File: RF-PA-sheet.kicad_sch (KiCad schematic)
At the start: 42 parts, among them J7 SMA_F, J8 U.fl, U10 MHW720A, U14 PSA4-5043, U17 B39431B3710U410

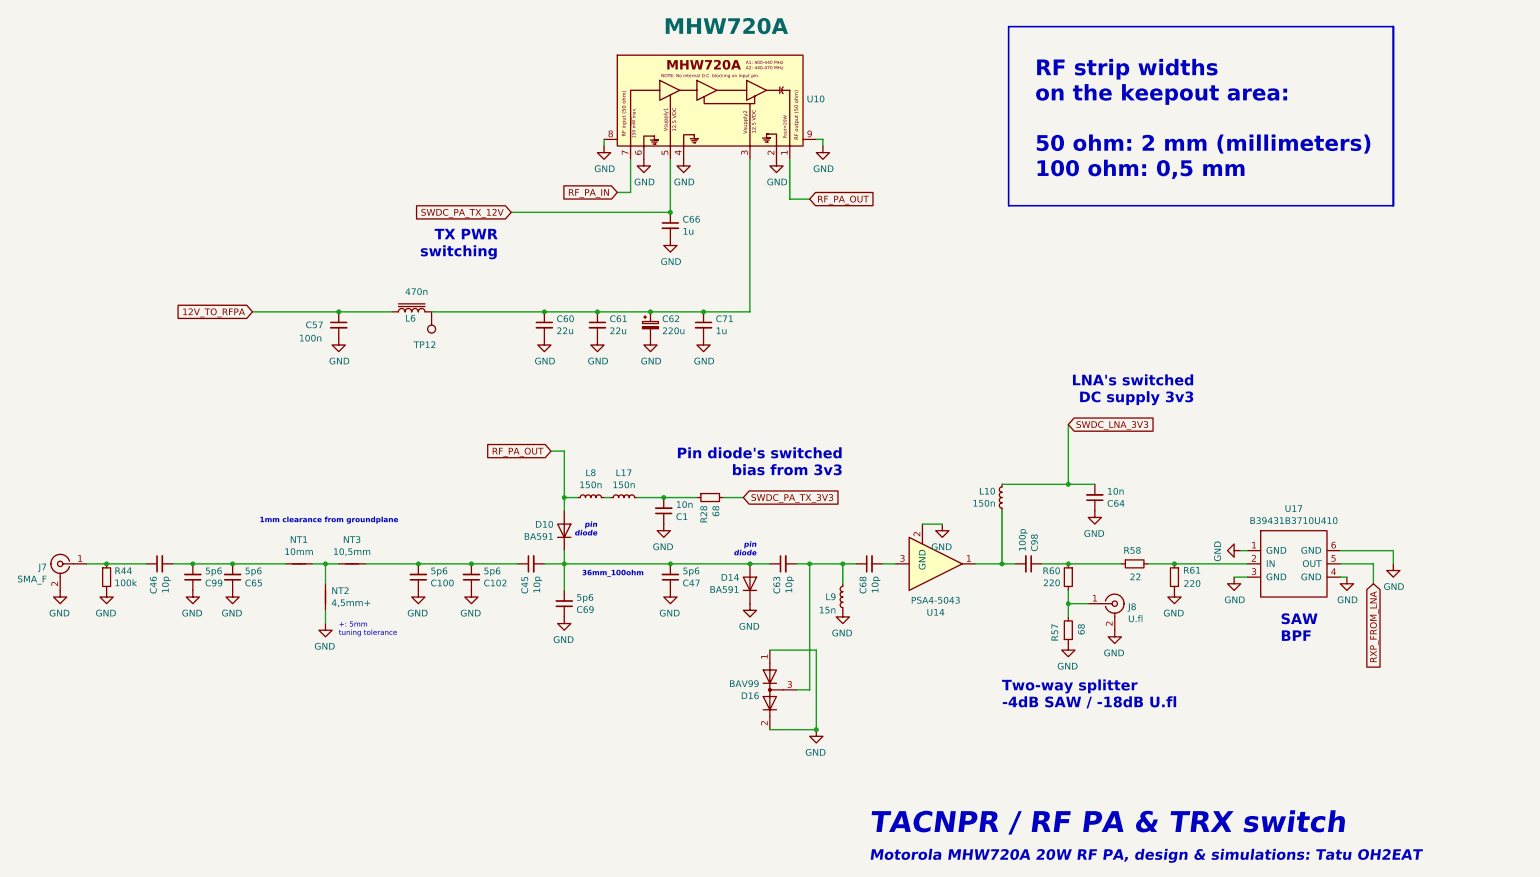
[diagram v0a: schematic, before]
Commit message: misc
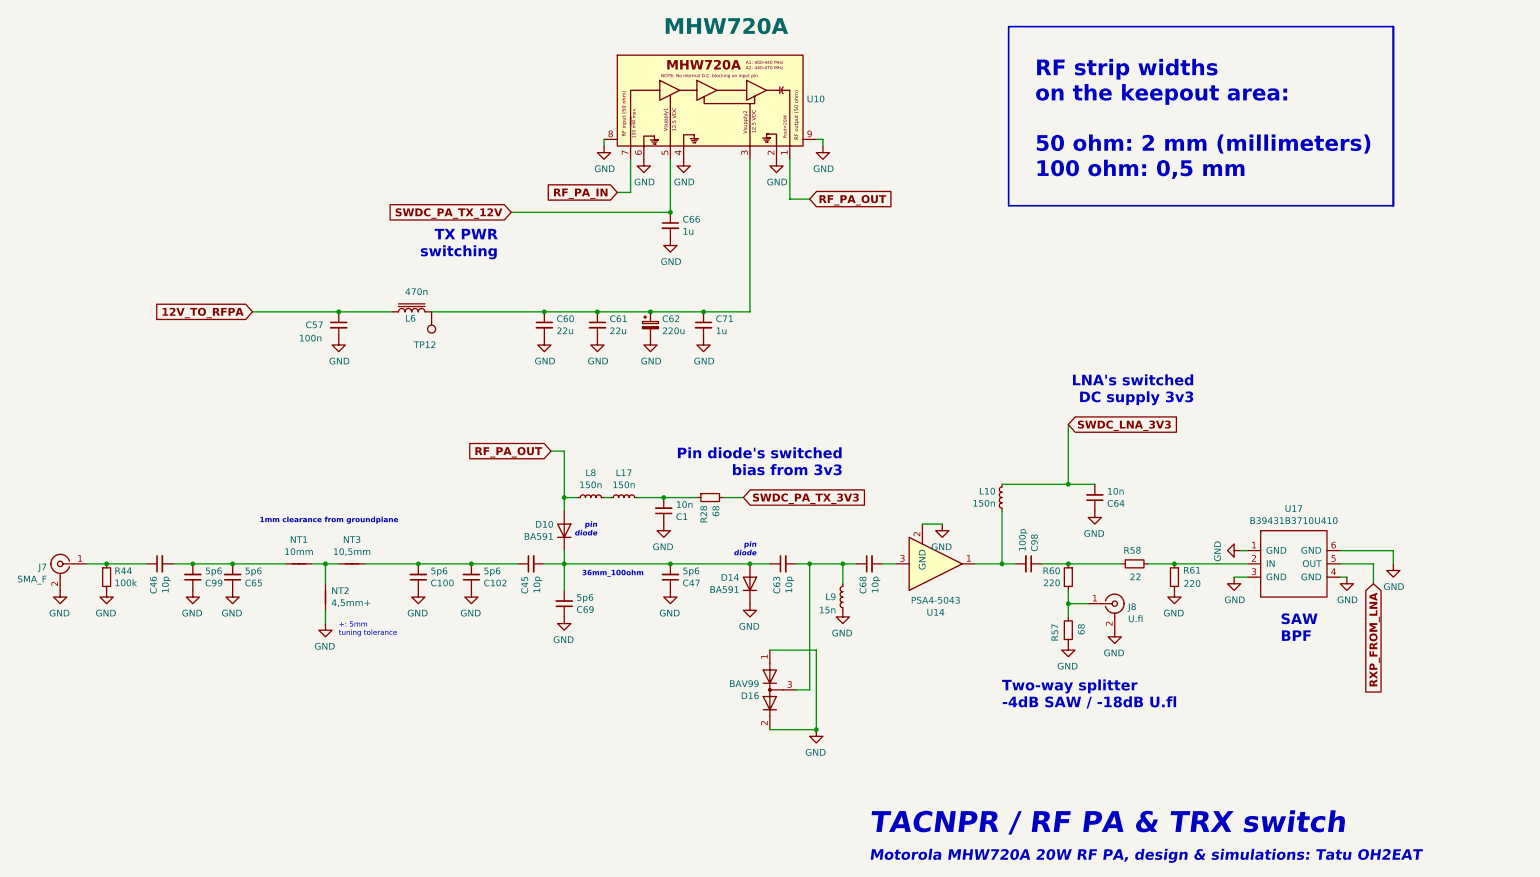
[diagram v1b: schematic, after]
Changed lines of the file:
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@@
   )
   (global_label "SWDC_PA_TX_12V" (shape input) (at 110.49 54.61 180) (fields_autoplaced)
-    (effects (font (size 1.27 1.27)) (justify right))
-    (property "Intersheet References" "${INTERSHEET_REFS}" (id 0) (at 0 0 0)
-      (effects (font (size 1.27 1.27)) hide)
+    (effects (font (size 1.5 1.5) (thickness 0.3) bold) (justify right))
+    (property "Intersheet References" "${INTERSHEET_REFS}" (id 0) (at 88.4486 54.46 0)
+      (effects (font (size 1.5 1.5) (thickness 0.3) bold) (justify right) hide)
     )
   )
   (global_label "SWDC_PA_TX_3V3" (shape input) (at 154.94 109.22 0) (fields_autoplaced)
-    (effects (font (size 1.27 1.27)) (justify left))
-    (property "Intersheet References" "${INTERSHEET_REFS}" (id 0) (at 0 0 0)
-      (effects (font (size 1.27 1.27)) hide)
+    (effects (font (size 1.5 1.5) (thickness 0.3) bold) (justify left))
+    (property "Intersheet References" "${INTERSHEET_REFS}" (id 0) (at 176.9814 109.07 0)
+      (effects (font (size 1.5 1.5) (thickness 0.3) bold) (justify left) hide)
     )
   )
   (global_label "RF_PA_OUT" (shape input) (at 167.64 52.07 0) (fields_autoplaced)
-    (effects (font (size 1.27 1.27)) (justify left))
-    (property "Intersheet References" "${INTERSHEET_REFS}" (id 0) (at 0 0 0)
-      (effects (font (size 1.27 1.27)) hide)
+    (effects (font (size 1.5 1.5) (thickness 0.3) bold) (justify left))
+    (property "Intersheet References" "${INTERSHEET_REFS}" (id 0) (at 182.7529 51.92 0)
+      (effects (font (size 1.5 1.5) (thickness 0.3) bold) (justify left) hide)
     )
   )
   (global_label "12V_TO_RFPA" (shape input) (at 60.96 73.66 180) (fields_autoplaced)
-    (effects (font (size 1.27 1.27)) (justify right))
-    (property "Intersheet References" "${INTERSHEET_REFS}" (id 0) (at 0 0 0)
-      (effects (font (size 1.27 1.27)) hide)
+    (effects (font (size 1.5 1.5) (thickness 0.3) bold) (justify right))
+    (property "Intersheet References" "${INTERSHEET_REFS}" (id 0) (at 43.2757 73.51 0)
+      (effects (font (size 1.5 1.5) (thickness 0.3) bold) (justify right) hide)
     )
   )
   (global_label "RXP_FROM_LNA" (shape input) (at 275.59 125.73 270) (fields_autoplaced)
-    (effects (font (size 1.27 1.27)) (justify right))
-    (property "Intersheet References" "${INTERSHEET_REFS}" (id 0) (at 0 0 0)
-      (effects (font (size 1.27 1.27)) hide)
+    (effects (font (size 1.5 1.5) (thickness 0.3) bold) (justify right))
+    (property "Intersheet References" "${INTERSHEET_REFS}" (id 0) (at 275.44 145.5571 90)
+      (effects (font (size 1.5 1.5) (thickness 0.3) bold) (justify right) hide)
     )
   )
   (global_label "SWDC_LNA_3V3" (shape input) (at 217.17 95.25 0) (fields_autoplaced)
-    (effects (font (size 1.27 1.27)) (justify left))
-    (property "Intersheet References" "${INTERSHEET_REFS}" (id 0) (at 0 0 0)
-      (effects (font (size 1.27 1.27)) hide)
+    (effects (font (size 1.5 1.5) (thickness 0.3) bold) (justify left))
+    (property "Intersheet References" "${INTERSHEET_REFS}" (id 0) (at 236.7829 95.1 0)
+      (effects (font (size 1.5 1.5) (thickness 0.3) bold) (justify left) hide)
     )
   )
   (global_label "RF_PA_IN" (shape input) (at 130.81 50.8 180) (fields_autoplaced)
-    (effects (font (size 1.27 1.27)) (justify right))
-    (property "Intersheet References" "${INTERSHEET_REFS}" (id 0) (at 0 0 0)
-      (effects (font (size 1.27 1.27)) hide)
+    (effects (font (size 1.5 1.5) (thickness 0.3) bold) (justify right))
+    (property "Intersheet References" "${INTERSHEET_REFS}" (id 0) (at 117.6971 50.65 0)
+      (effects (font (size 1.5 1.5) (thickness 0.3) bold) (justify right) hide)
     )
   )
   (global_label "RF_PA_OUT" (shape input) (at 118.11 100.33 180) (fields_autoplaced)
-    (effects (font (size 1.27 1.27)) (justify right))
-    (property "Intersheet References" "${INTERSHEET_REFS}" (id 0) (at 0 0 0)
-      (effects (font (size 1.27 1.27)) hide)
+    (effects (font (size 1.5 1.5) (thickness 0.3) bold) (justify right))
+    (property "Intersheet References" "${INTERSHEET_REFS}" (id 0) (at 102.9971 100.18 0)
+      (effects (font (size 1.5 1.5) (thickness 0.3) bold) (justify right) hide)
     )
   )
